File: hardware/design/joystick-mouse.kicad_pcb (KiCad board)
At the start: 2 copper layers, 9 parts

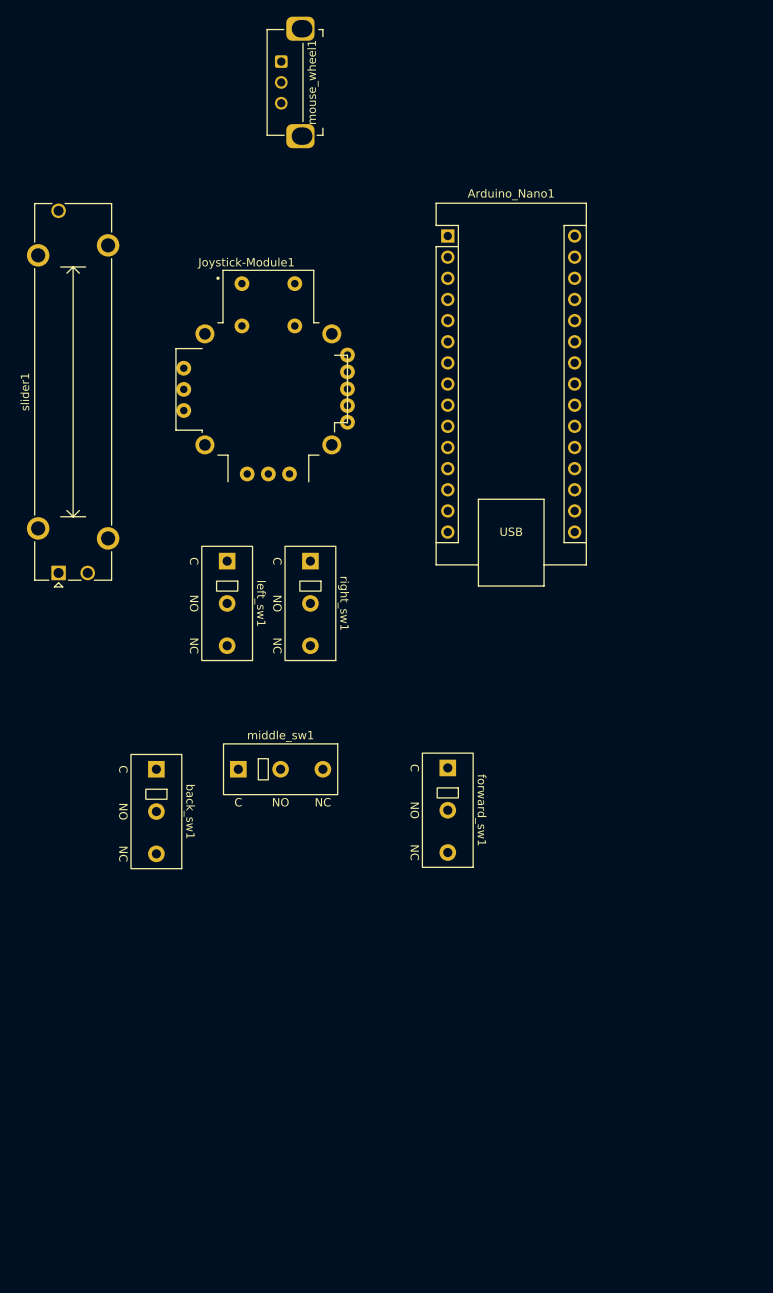
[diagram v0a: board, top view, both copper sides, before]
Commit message: finish pcb
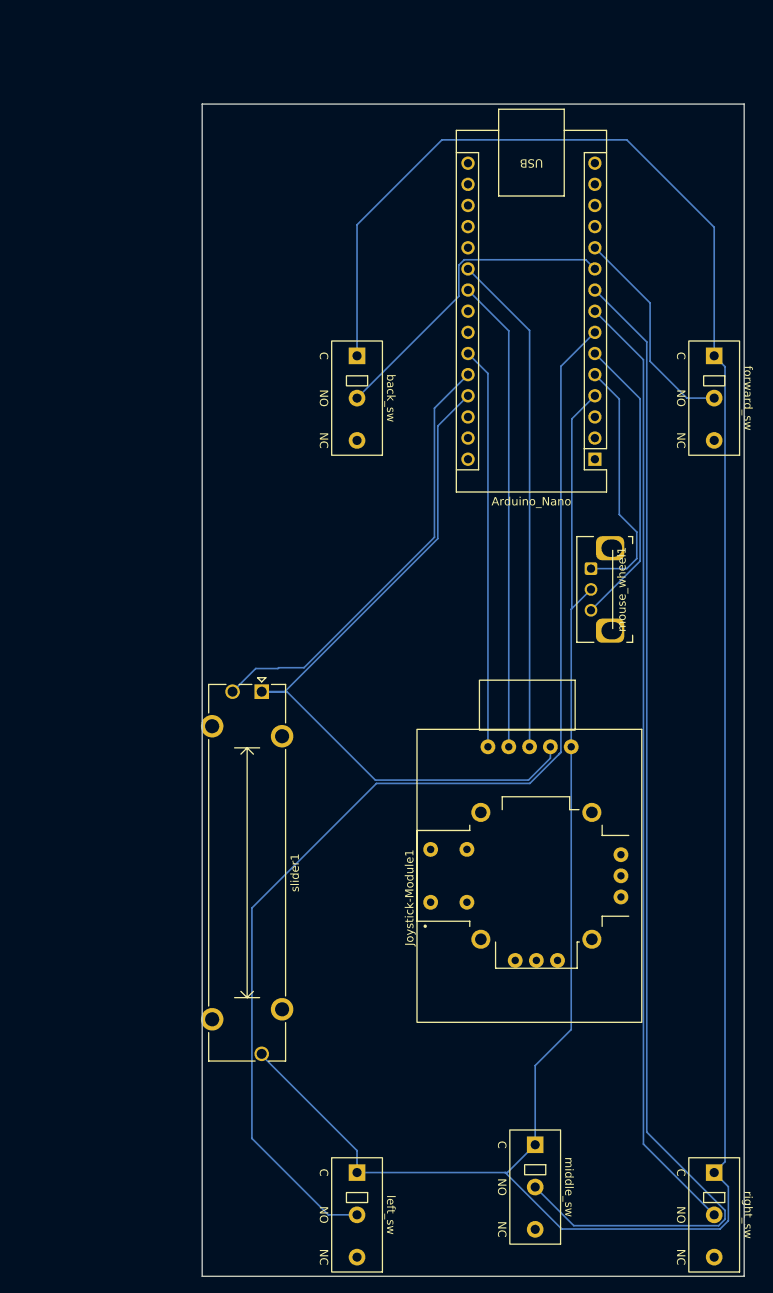
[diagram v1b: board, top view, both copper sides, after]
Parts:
- Joystick-Module1: footprint COM-09032:XDCR_COM-09032 -> ky-023_joystick:ky-023_joystick
- moved right_sw 88.0 mm to (162.0, 158.4)
- moved left_sw 75.1 mm to (119.1, 158.4)
- moved mouse_wheel1 71.4 mm to (147.2, 85.9)
- moved Joystick-Module1 66.8 mm to (140.8, 122.8), turned to -90 degrees
- moved forward_sw 58.9 mm to (162.0, 60.3)
- moved middle_sw 57.5 mm to (140.5, 155.1), turned to -90 degrees
- moved back_sw 55.2 mm to (119.1, 60.3)
- moved Arduino_Nano 32.1 mm to (147.7, 72.8), turned to 180 degrees
- moved slider1 28.3 mm to (107.7, 100.7), turned to -90 degrees
- renumbered Arduino_Nano1 to Arduino_Nano, back_sw1 to back_sw, forward_sw1 to forward_sw, left_sw1 to left_sw, middle_sw1 to middle_sw, right_sw1 to right_sw
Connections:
- Arduino_Nano pad 19: Net-(Arduino_Nano1-A0) -> unconnected-(Arduino_Nano1-A0-Pad19)
- Arduino_Nano pad 25: unconnected-(Arduino_Nano1-A6-Pad25) -> Net-(Arduino_Nano1-A6)
- Arduino_Nano pad 26: unconnected-(Arduino_Nano1-A7-Pad26) -> Net-(Arduino_Nano1-A7)
- forward_sw pad 2: Net-(Arduino_Nano1-D6) -> Net-(Arduino_Nano1-D8)
- middle_sw pad 2: Net-(Arduino_Nano1-D8) -> Net-(Arduino_Nano1-D6)
- slider1 pad 2: Net-(Arduino_Nano1-A0) -> Net-(Arduino_Nano1-A7)
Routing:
- net GND: track 0.00 -> 356.3 mm
- net Net-(Arduino_Nano1-D6): track 0.00 -> 143.1 mm
- net Net-(Arduino_Nano1-D4): track 0.00 -> 141.5 mm
- net Net-(Arduino_Nano1-D5): track 0.00 -> 114.6 mm
- net +5V: track 0.00 -> 89.0 mm
- net Net-(Arduino_Nano1-A2): track 0.00 -> 60.5 mm
- net Net-(Arduino_Nano1-A3): track 0.00 -> 56.9 mm
- net Net-(Arduino_Nano1-A7): track 0.00 -> 53.1 mm
- net Net-(Arduino_Nano1-A6): track 0.00 -> 48.2 mm
- net Net-(Arduino_Nano1-D7): track 0.00 -> 38.1 mm
- net Net-(Arduino_Nano1-D3): track 0.00 -> 35.5 mm
- net Net-(Arduino_Nano1-D2): track 0.00 -> 30.2 mm
- net Net-(Arduino_Nano1-D8): track 0.00 -> 25.9 mm
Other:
- board outline added: 65.1 x 140.8 mm
